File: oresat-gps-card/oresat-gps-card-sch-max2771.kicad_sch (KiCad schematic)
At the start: 78 parts, among them U12 7Q-16.368MBG-T, U13 MAX2769, U20 MAX2769ETI+, U21 LT1719S6, U22 XC2C64A-5VQG44C, U24 D32G-016.368M, U26 LT1719IS6, U28 LT1719IS6

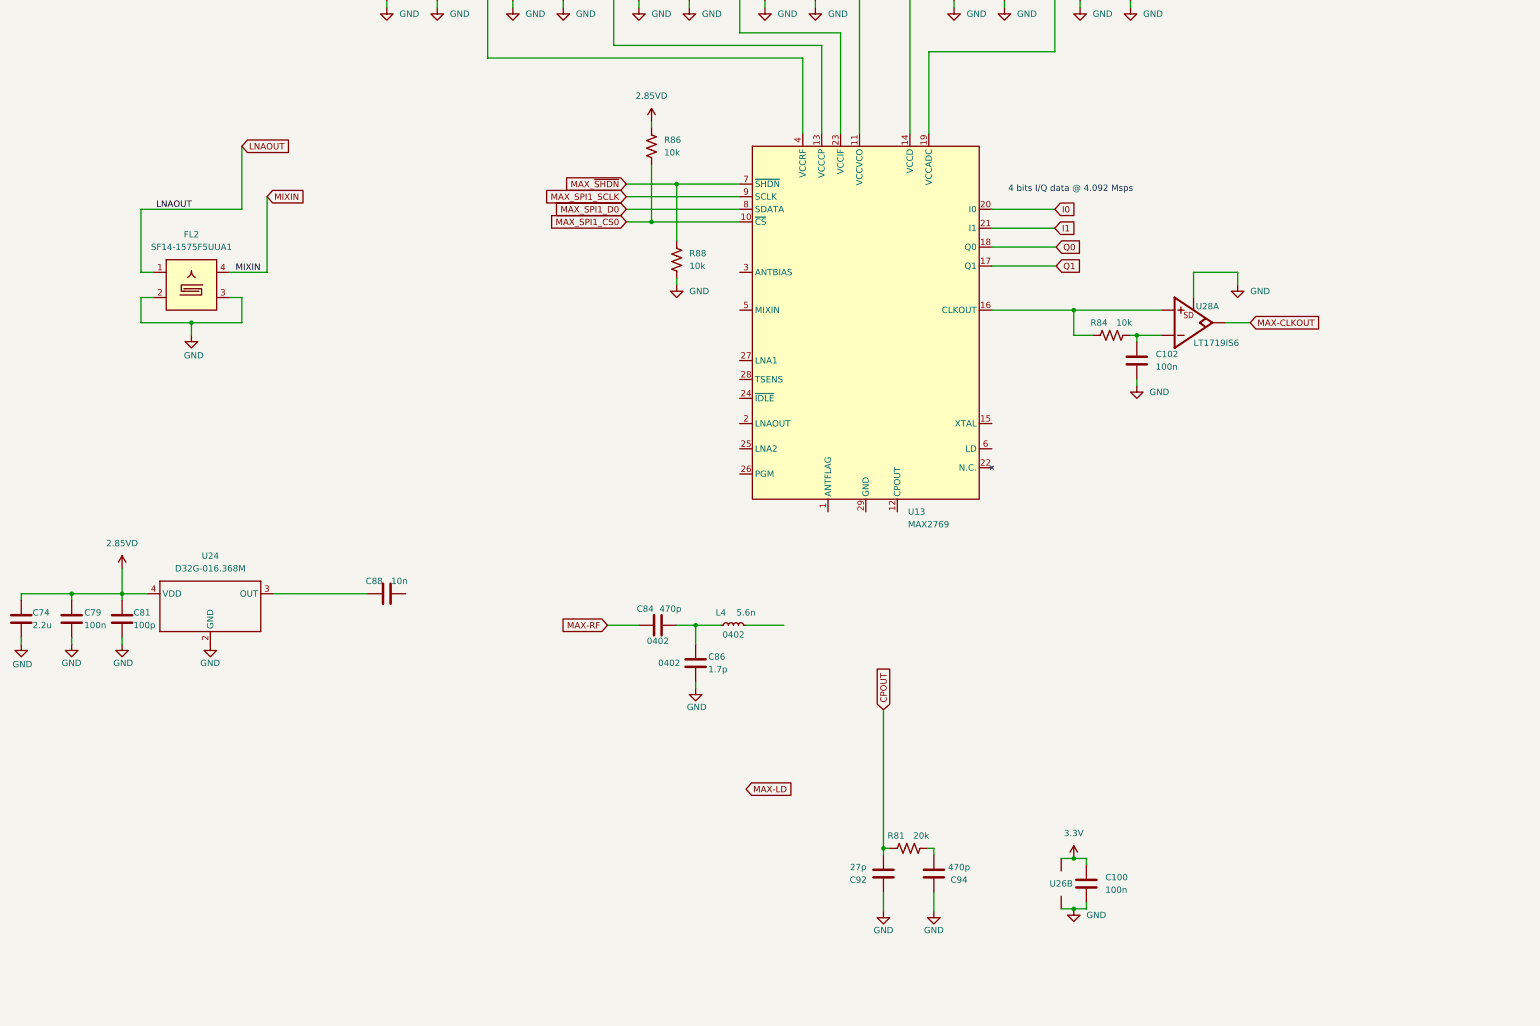
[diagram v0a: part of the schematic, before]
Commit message: Routine Push
Andrew should look at the MAX2769 change.
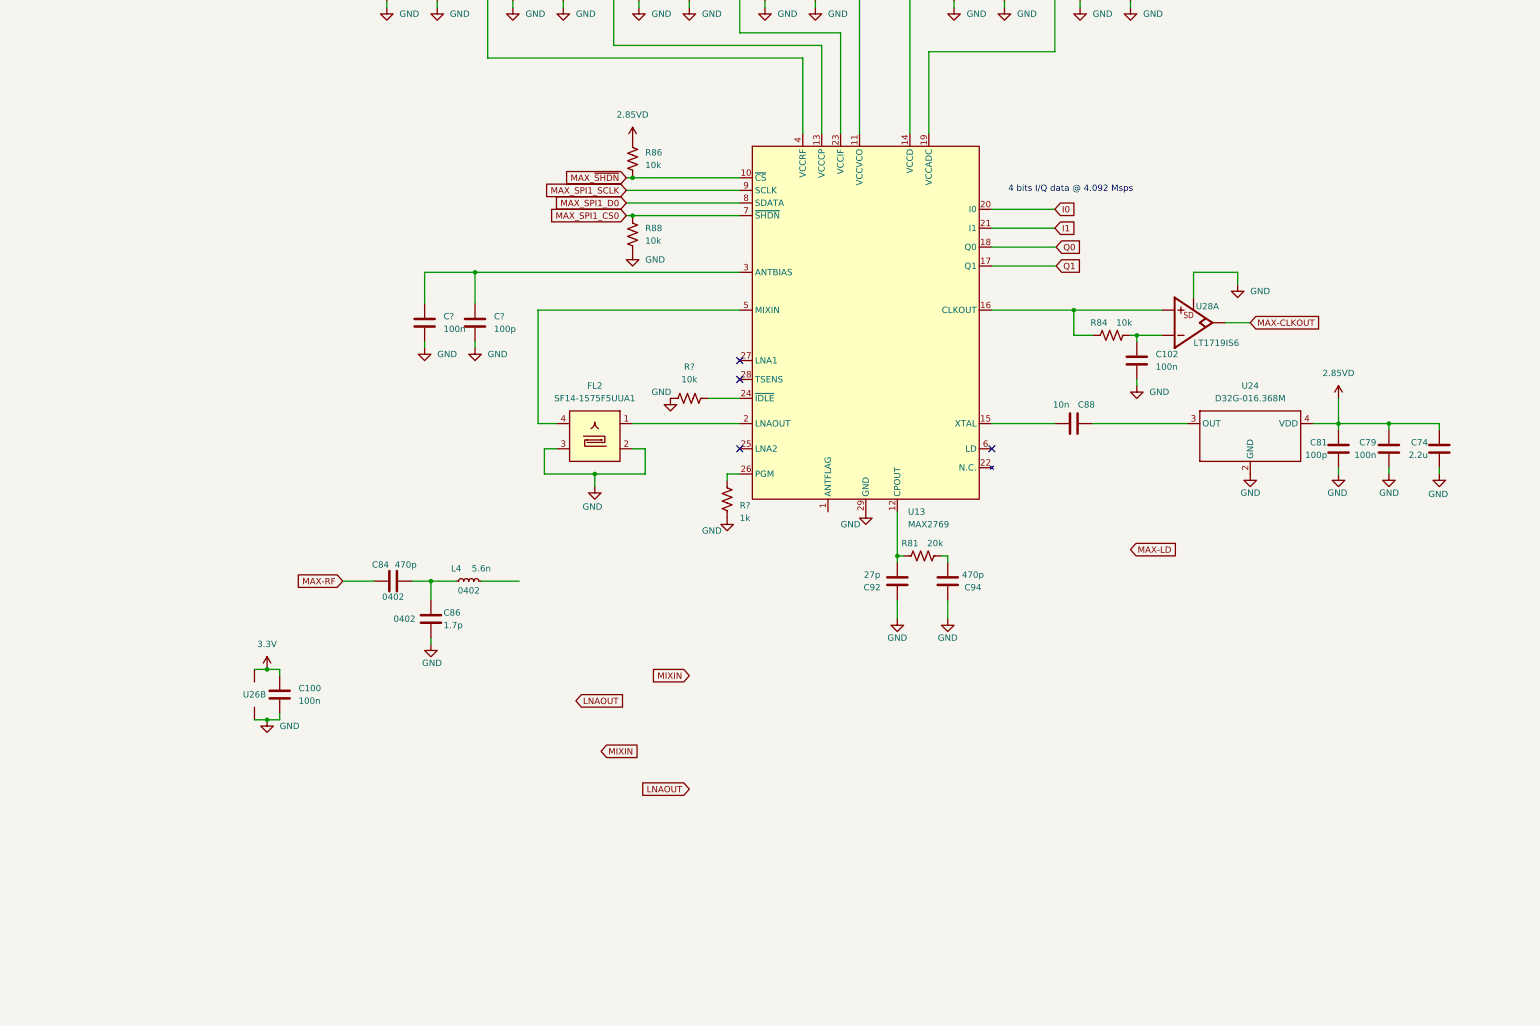
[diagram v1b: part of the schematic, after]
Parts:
- added C?: 100p, Capacitor_SMD:C_0603_1608Metric, symbol Device:C
- added C?: 100n, Capacitor_SMD:C_0603_1608Metric, symbol Device:C
- added R?: 1k, Resistor_SMD:R_0603_1608Metric, symbol Device:R_US
- added R?: 10k, Resistor_SMD:R_0603_1608Metric, symbol Device:R_US
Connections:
- net CPOUT is gone; now on an unnamed net: C92.2, R81.2
- net GND: now also U13.29 (GND), C?.2, C?.2, R?.1, R?.2
- net LNAOUT: no longer FL2.1
- net MAX_SPI1_CS0: now also R88.1, U13.7 (~{SHDN}); no longer R86.2, U13.10 (~{CS})
- net MAX_~{SHDN}: now also R86.2, U13.10 (~{CS}); no longer R88.1, U13.7 (~{SHDN})
- net MIXIN: no longer FL2.4
- net at U13.15 (XTAL): now also C88.2
- net at U13.2 (LNAOUT): now also FL2.1
- net at U13.24 (~{IDLE}): now also R?.2
- net at U13.26 (PGM): now also R?.1
- net at U13.3 (ANTBIAS): now also C?.1, C?.1
- net at U13.5 (MIXIN): now also FL2.4
- no-connect marks 0 -> 4
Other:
- moved on the sheet: C100, C74, C79, C81, C84, C86, C88, C92, C94, FL2, L4, R81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
